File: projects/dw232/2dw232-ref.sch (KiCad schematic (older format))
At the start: 25 parts, among them Q501 MMBT3904, Q502 MMBT3904, U501 LM741, U502 LM741, U503 2DW232

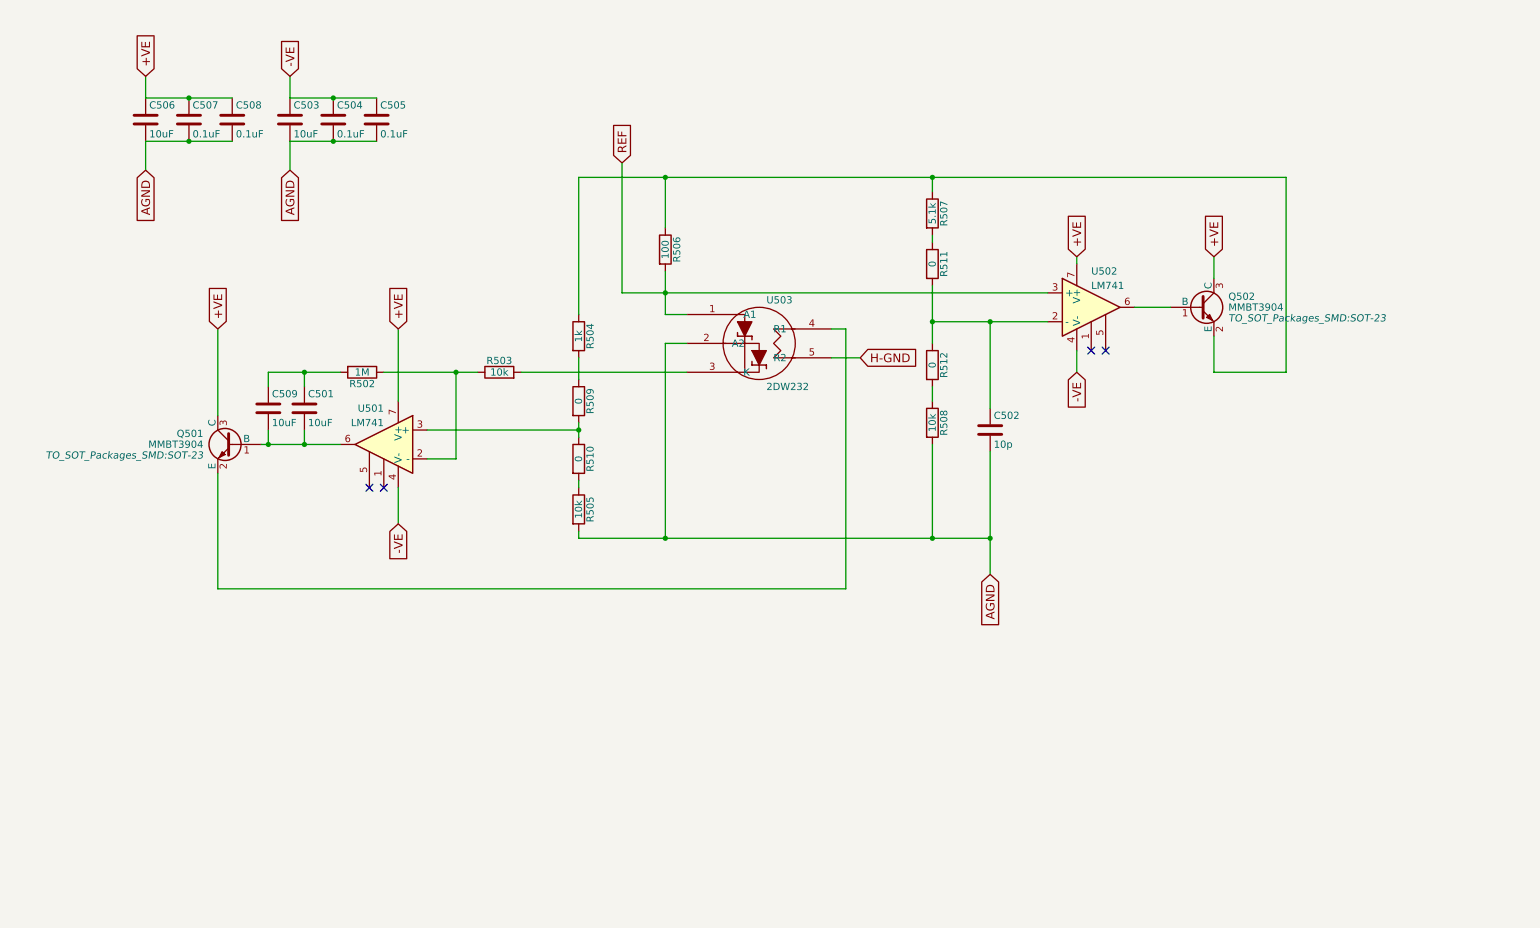
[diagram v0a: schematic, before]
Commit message: update
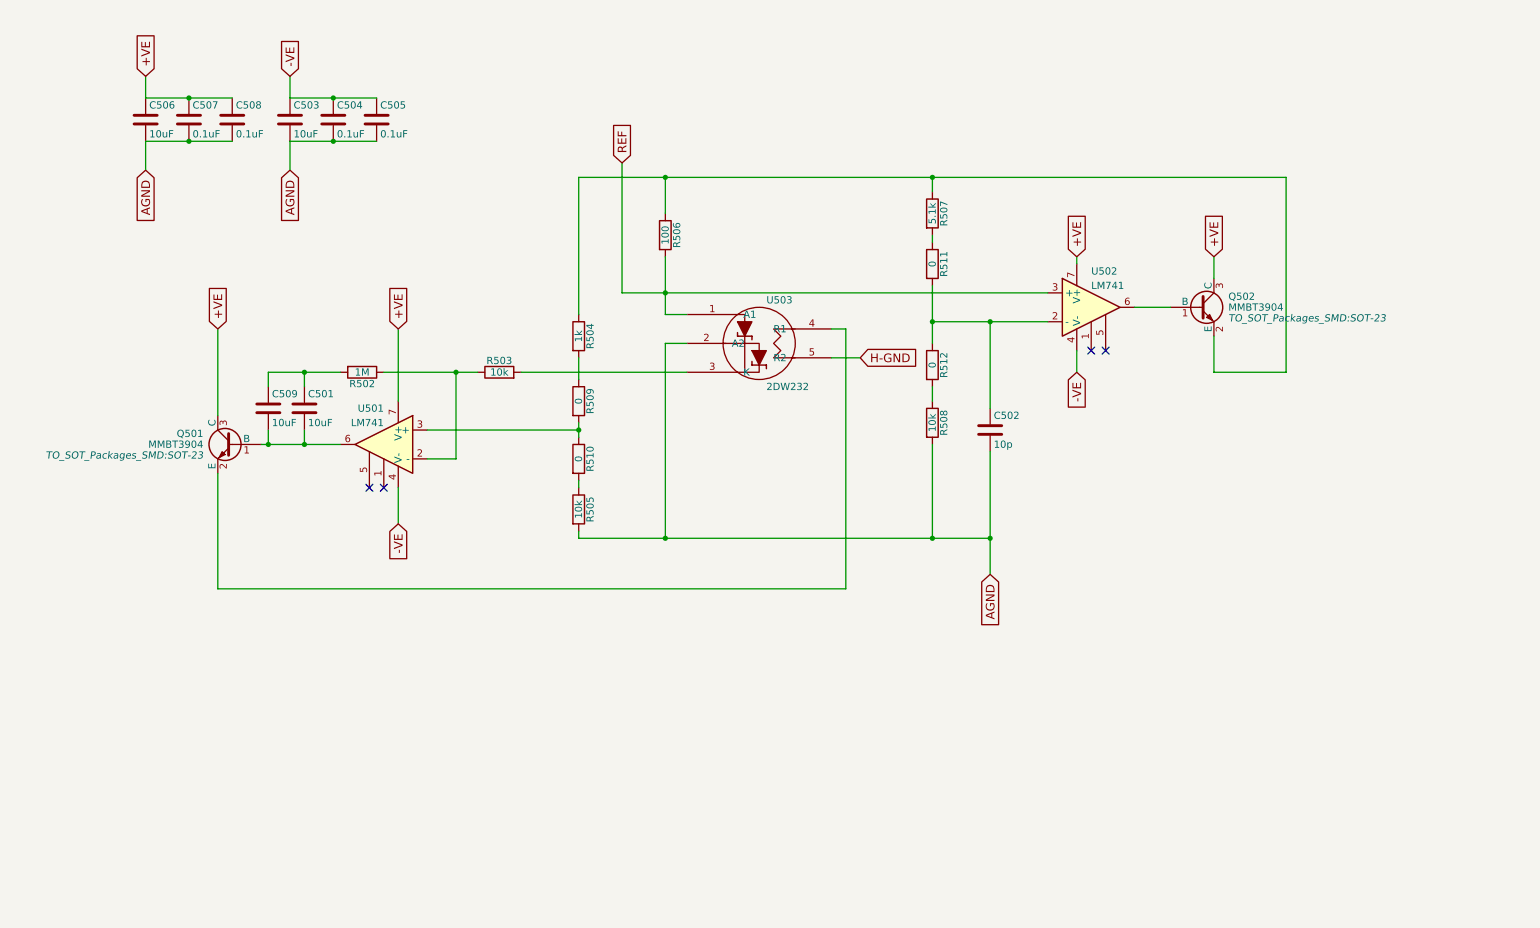
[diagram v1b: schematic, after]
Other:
- moved on the sheet: R506
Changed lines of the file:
@@
 $EndComp
 Wire Wire Line
-	3850 1650 4450 1650
-Wire Wire Line
-	4450 1650 6300 1650
-Wire Wire Line
-	6300 1650 8750 1650
+	3850 1650 8750 1650
 Wire Wire Line
 	6300 1650 6300 1750
 Wire Wire Line
-	6300 2400 6300 2650
-Wire Wire Line
-	6300 2650 6300 2800
+	6300 2400 6300 2800
 Text GLabel 7300 2200 1    60   Input ~ 0
 +VE
@@
 AGND
 Wire Wire Line
-	6300 2650 6700 2650
-Wire Wire Line
-	6700 2650 7100 2650
+	6300 2650 7100 2650
 Connection ~ 6300 2650
 Wire Wire Line
-	4150 2450 4450 2450
-Wire Wire Line
-	4450 2450 7100 2450
-Wire Wire Line
-	3850 4150 4450 4150
-Wire Wire Line
-	4450 4150 6300 4150
-Wire Wire Line
-	6300 4150 6700 4150
+	4150 2450 7100 2450
+Wire Wire Line
+	3850 4150 6700 4150
 Connection ~ 6300 4150
 $Comp
 L R R506
 U 1 1 5881872C
-P 4450 2150
-F 0 "R506" V 4530 2150 50  0000 C CNN
-F 1 "100" V 4450 2150 50  0000 C CNN
-F 2 "Resistors_ThroughHole:Resistor_TO-220_Vertical" V 4380 2150 50  0001 C CNN
-F 3 "" H 4450 2150 50  0000 C CNN
-	1    4450 2150
+P 4450 2050
+F 0 "R506" V 4530 2050 50  0000 C CNN
+F 1 "100" V 4450 2050 50  0000 C CNN
+F 2 "Resistors_ThroughHole:Resistor_TO-220_Vertical" V 4380 2050 50  0001 C CNN
+F 3 "" H 4450 2050 50  0000 C CNN
+	1    4450 2050
 	1    0    0    -1
 $EndComp
@@
 $EndComp
 Wire Wire Line
-	2500 3000 3000 3000
-Wire Wire Line
-	3000 3000 3150 3000
+	2500 3000 3150 3000
 Wire Wire Line
 	3000 3000 3000 3600
@@
 $EndComp
 Wire Wire Line
-	1700 3000 1950 3000
-Wire Wire Line
-	1950 3000 2200 3000
+	1700 3000 2200 3000
 Wire Wire Line
 	1950 3000 1950 3100
 Wire Wire Line
-	1950 3400 1950 3500
-Wire Wire Line
-	1650 3500 1700 3500
-Wire Wire Line
-	1700 3500 1950 3500
-Wire Wire Line
-	1950 3500 2200 3500
+	1950 3500 1950 3400
+Wire Wire Line
+	1650 3500 2200 3500
 Text GLabel 2600 2700 1    60   Input ~ 0
 +VE
@@
 	3850 4100 3850 4150
 Wire Wire Line
-	6700 3550 6700 4150
-Wire Wire Line
-	6700 4150 6700 4400
+	6700 3550 6700 4400
 Connection ~ 6700 4150
 Wire Wire Line
@@
 	1850 950  1850 1100
 Wire Wire Line
-	1850 1100 2150 1100
-Wire Wire Line
-	2150 1100 2450 1100
-Wire Wire Line
-	1850 1400 2150 1400
-Wire Wire Line
-	2150 1400 2450 1400
+	1850 1100 2450 1100
+Wire Wire Line
+	1850 1400 2450 1400
 Connection ~ 2150 1100
 Connection ~ 2150 1400
@@
 	4450 2600 4600 2600
 Wire Wire Line
-	4450 2300 4450 2450
-Wire Wire Line
-	4450 2450 4450 2600
-Wire Wire Line
-	4450 1650 4450 2000
+	4450 2200 4450 2600
+Wire Wire Line
+	4450 1650 4450 1900
 Connection ~ 4450 1650
 Connection ~ 4450 2450
@@
 	850  950  850  1100
 Wire Wire Line
-	850  1100 1150 1100
-Wire Wire Line
-	1150 1100 1450 1100
-Wire Wire Line
-	850  1400 1150 1400
-Wire Wire Line
-	1150 1400 1450 1400
+	850  1100 1450 1100
+Wire Wire Line
+	850  1400 1450 1400
 Connection ~ 1150 1100
 Connection ~ 1150 1400
@@
 	3850 3750 3850 3800
 Wire Wire Line
-	3850 3350 3850 3400
-Wire Wire Line
-	3850 3400 3850 3450
+	3850 3350 3850 3450
 Wire Wire Line
 	3850 3400 2800 3400

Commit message: v0.2 2dw232
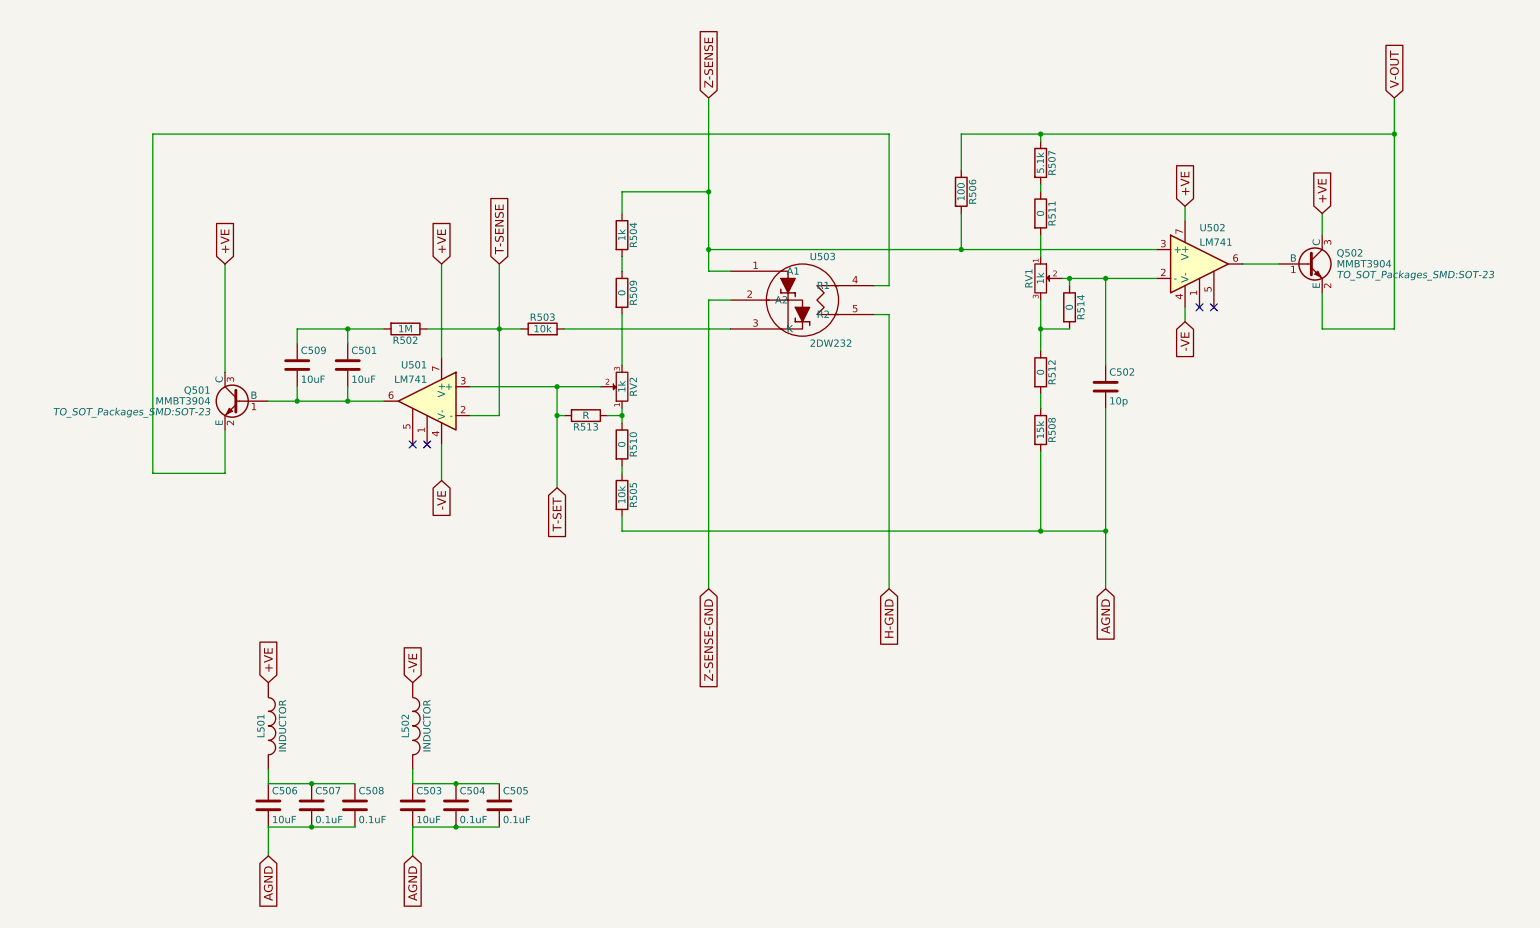
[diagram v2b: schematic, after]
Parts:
- added L501, L502: INDUCTOR, symbol INDUCTOR
- added R513: R, symbol R
- added R514: 0, Resistors_ThroughHole:Resistor_TO-220_Vertical, symbol R
- added RV1, RV2: 1k, symbol POT
- R508: value 10k -> 15k
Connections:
- net +VE: now also L501.1; no longer C506.1, C507.1, C508.1
- net -VE: now also L502.1; no longer C503.1, C504.1, C505.1
- net AGND: no longer U503.2 (A2)
- net at C502.1, U502.2 (-): now also R514.1, RV1.2; no longer R511.2, R512.1
- net V-OUT: now reaches Q502.2 (E), R506.1, R507.1
- net V-OUT: no longer R504.1
- net T-SENSE: now reaches R502.1, R503.1, U501.2 (-)
- net REF renamed Z-SENSE
- net Z-SENSE: now also R504.1
- new net: C503.1, C504.1, C505.1, L502.2
- new net: C506.1, C507.1, C508.1, L501.2
- new net: R510.1, R513.1, RV2.1
- new net: R509.2, RV2.3
- new net: R512.1, R514.2, RV1.3
- new net: R511.2, RV1.1
- new net T-SET: R513.2, RV2.2, U501.3 (+)
- new net Z-SENSE-GND: U503.2 (A2)
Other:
- moved on the sheet: C501, C502, C503, C504, C505, C506, C507, C508, C509, Q501, Q502, R502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
